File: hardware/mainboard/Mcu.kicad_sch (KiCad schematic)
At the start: 12 parts, among them U10 STM32H573RITx

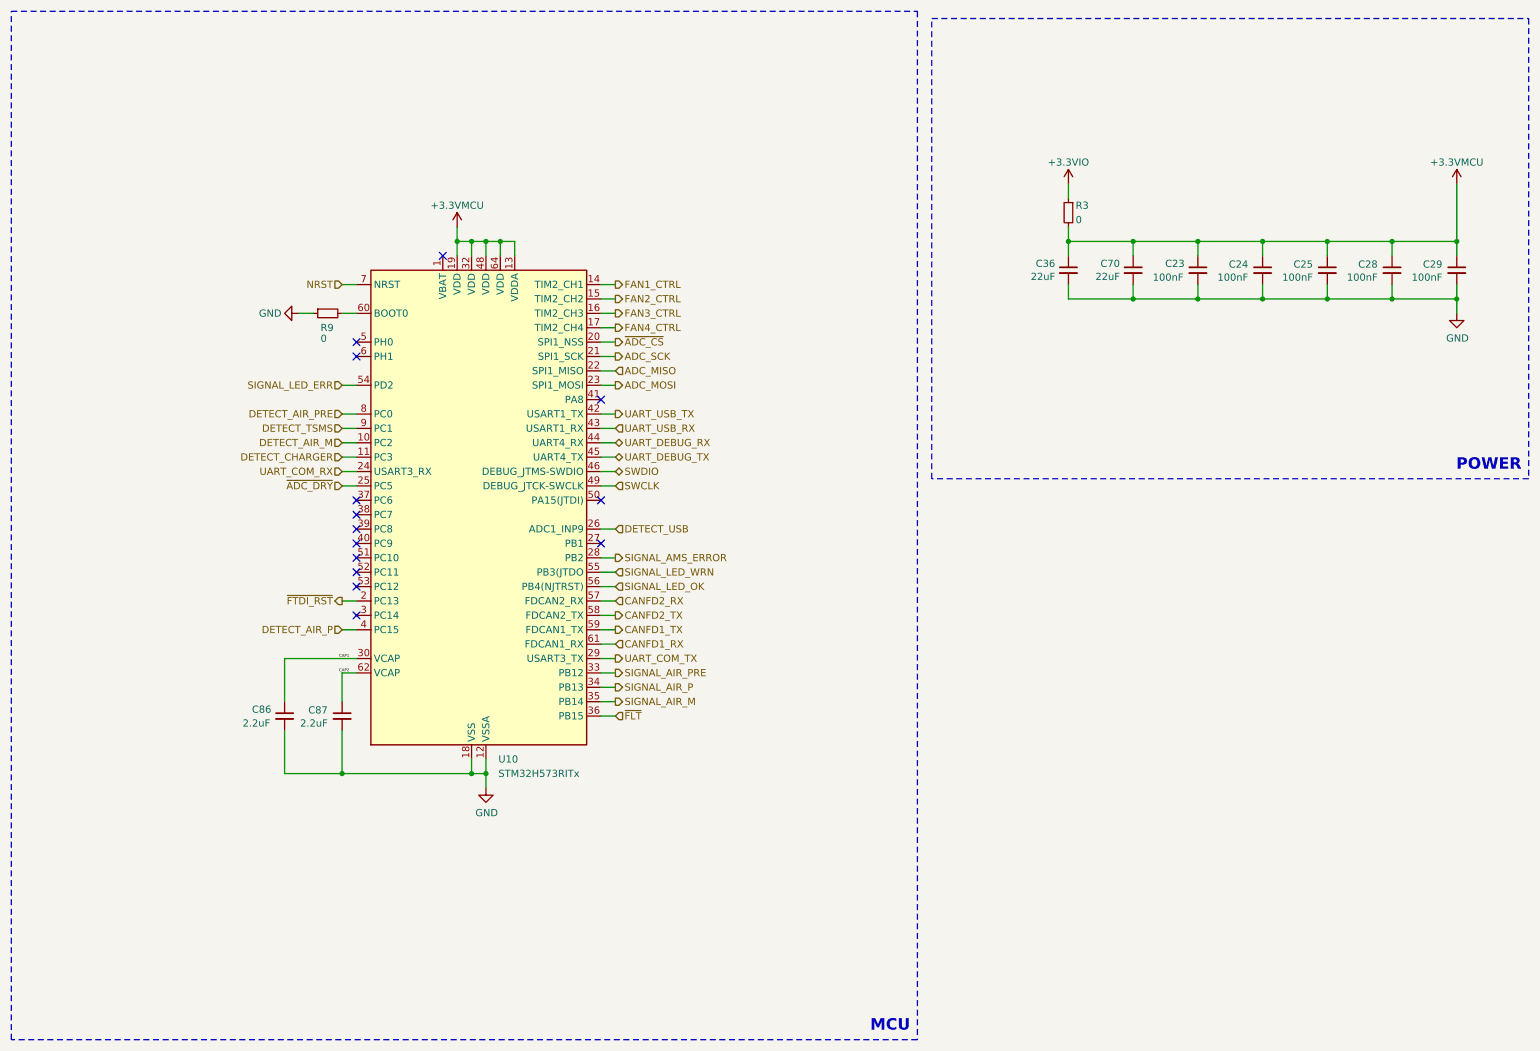
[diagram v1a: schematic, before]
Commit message: Layout ver.2
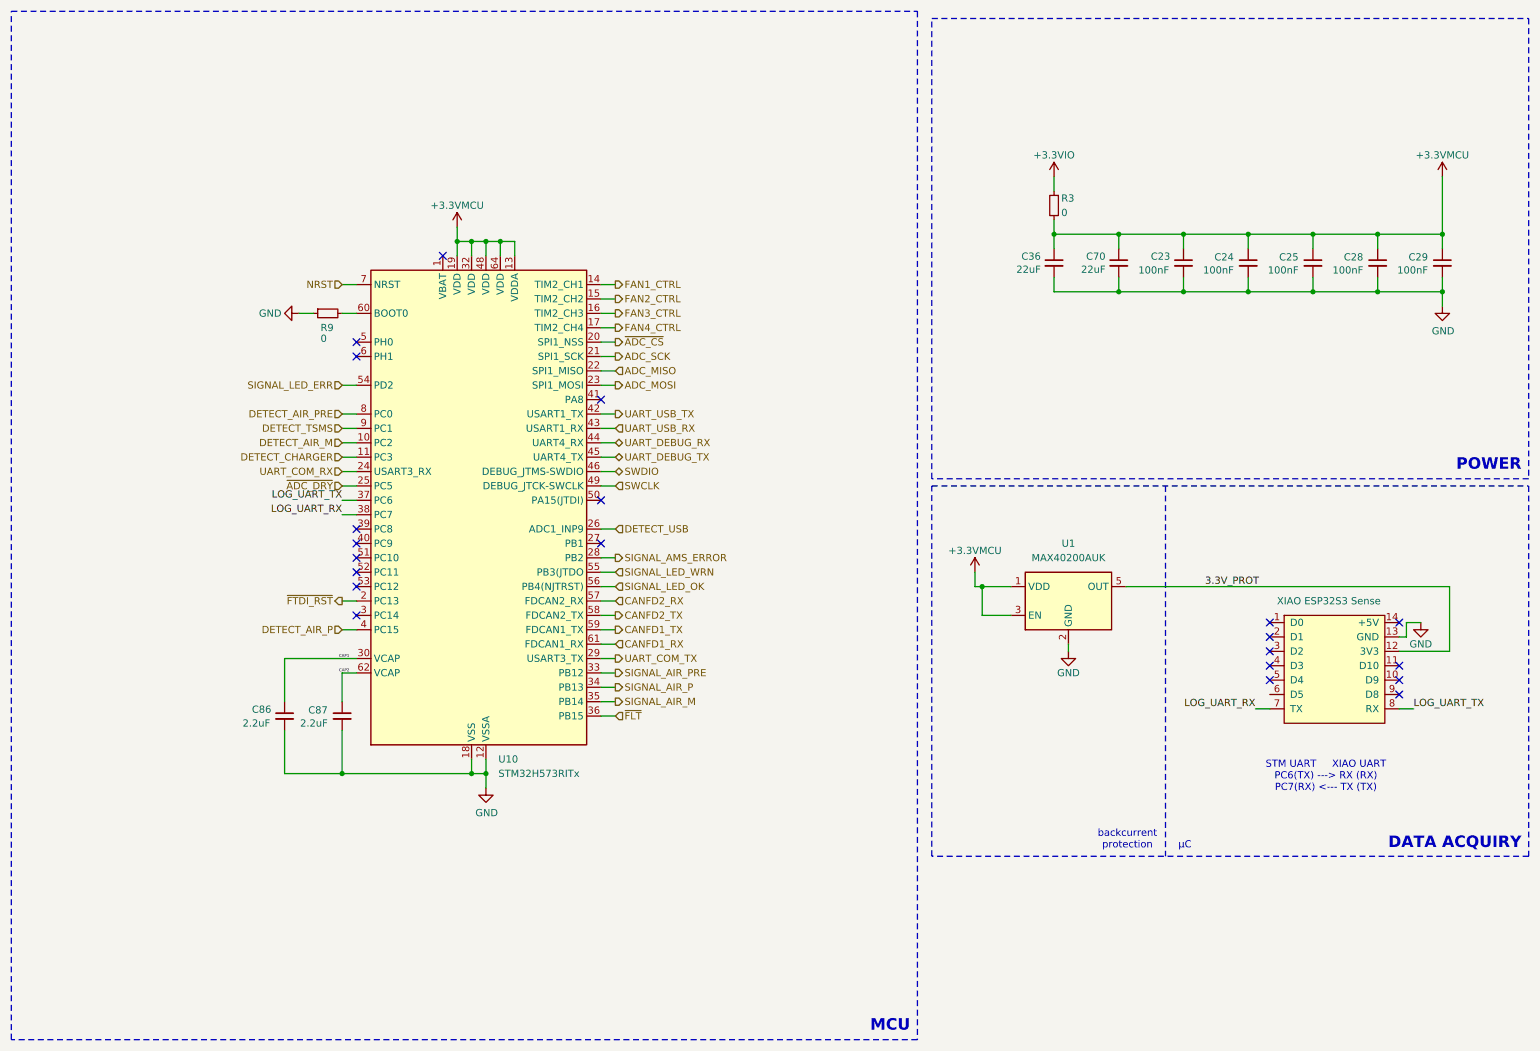
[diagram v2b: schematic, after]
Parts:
- added J2: XIAO ESP32S3 Sense, xiao:XIAO-ESP32-S3-DIP, symbol Connector:Conn_01x04_Socket
- added U1: MAX40200AUK, Package_TO_SOT_SMD:SOT-23-5_HandSoldering, symbol Analog_Switch:MAX40200AUK
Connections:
- net +3.3VMCU: now also U1.1 (VDD), U1.3 (EN)
- net GND: now also J2.13 (GND), U1.2 (GND)
- net LOG_UART_TX: now reaches U10.37 (PC6)
- net LOG_UART_TX: now also J2.8 (RX)
- net LOG_UART_RX: now reaches U10.38 (PC7)
- net LOG_UART_RX: now also J2.7 (TX)
- new net 3.3V_PROT: J2.12 (3V3), U1.5 (OUT)
- no-connect marks 14 -> 21
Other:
- note added: "DATA ACQUIRY"
- note added: "STM UART XIAO UART PC6(TX) ---> RX (RX) PC7(RX) <--- TX (TX)"
- note added: "backcurrent protection"
- note added: "μC"
- moved on the sheet: C23, C24, C25, C28, C29, C36, C70, R3
